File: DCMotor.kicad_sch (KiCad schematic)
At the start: 18 parts, among them J10 Conn_01x03_Socket, J11 Conn_01x02_Socket, J12 Conn_01x03_Socket, J13 Conn_01x03_Socket, J14 Conn_01x03_Socket, J7 Conn_01x02_Socket, J8 Conn_01x03_Socket, J9 Conn_01x02_Socket

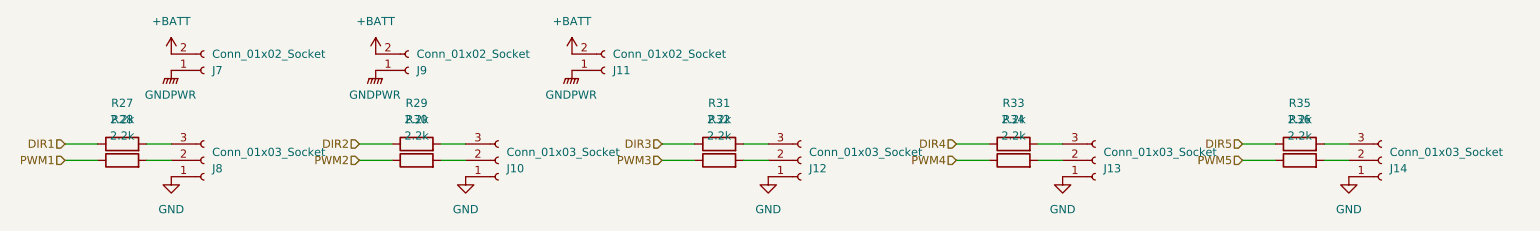
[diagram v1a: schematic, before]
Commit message: before elimination of J7
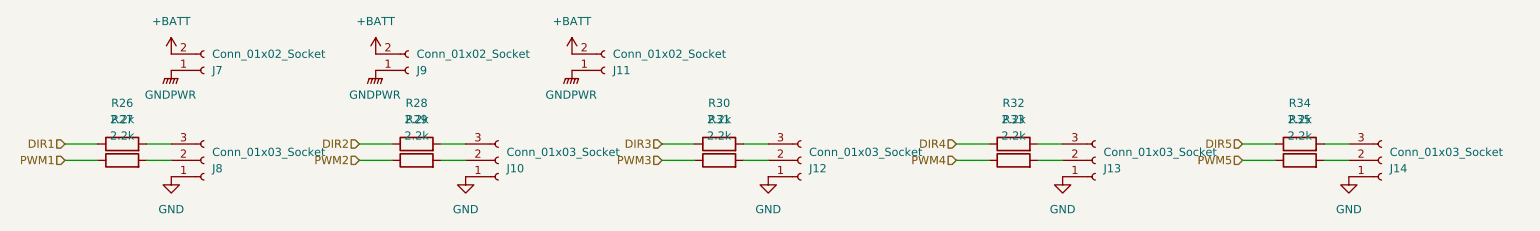
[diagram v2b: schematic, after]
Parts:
- renumbered R27 to R26, R28 to R27, R29 to R28, R30 to R29, R31 to R30, R32 to R31, R33 to R32, R34 to R33, R35 to R34, R36 to R35
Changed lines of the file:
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@@
 		(dnp no)
 		(fields_autoplaced yes)
-		(property "Reference" "R34"
+		(property "Reference" "R33"
 			(at 171.45 52.07 90)
 			(effects
@@
 			(project "chibarobo_board_2024"
 				(path "/7933aef9-9608-4ce1-b0d8-a4ffd3b998e4/10a4ce65-96c0-4b0e-ad7d-0749d3a88abd"
-					(reference "R34")
+					(reference "R33")
 					(unit 1)
 				)
@@
 		(dnp no)
 		(fields_autoplaced yes)
-		(property "Reference" "#PWR055"
+		(property "Reference" "#PWR054"
 			(at 72.39 49.53 0)
 			(effects
@@
 			(project "chibarobo_board_2024"
 				(path "/7933aef9-9608-4ce1-b0d8-a4ffd3b998e4/10a4ce65-96c0-4b0e-ad7d-0749d3a88abd"
-					(reference "#PWR055")
+					(reference "#PWR054")
 					(unit 1)
 				)
@@
 		(dnp no)
 		(fields_autoplaced yes)
-		(property "Reference" "#PWR052"
+		(property "Reference" "#PWR051"
 			(at 40.64 49.53 0)
 			(effects
@@
 			(project ""
 				(path "/7933aef9-9608-4ce1-b0d8-a4ffd3b998e4/10a4ce65-96c0-4b0e-ad7d-0749d3a88abd"
-					(reference "#PWR052")
+					(reference "#PWR051")
 					(unit 1)
 				)
@@
 		(dnp no)
 		(fields_autoplaced yes)
-		(property "Reference" "#PWR051"
+		(property "Reference" "#PWR050"
 			(at 40.64 45.72 0)
 			(effects
@@
 			(project ""
 				(path "/7933aef9-9608-4ce1-b0d8-a4ffd3b998e4/10a4ce65-96c0-4b0e-ad7d-0749d3a88abd"
-					(reference "#PWR051")
+					(reference "#PWR050")
 					(unit 1)
 				)
@@
 		(dnp no)
 		(fields_autoplaced yes)
-		(property "Reference" "R32"
+		(property "Reference" "R31"
 			(at 125.73 52.07 90)
 			(effects
@@
 			(project "chibarobo_board_2024"
 				(path "/7933aef9-9608-4ce1-b0d8-a4ffd3b998e4/10a4ce65-96c0-4b0e-ad7d-0749d3a88abd"
-					(reference "R32")
+					(reference "R31")
 					(unit 1)
 				)
@@
 		(dnp no)
 		(fields_autoplaced yes)
-		(property "Reference" "R31"
+		(property "Reference" "R30"
 			(at 125.73 49.53 90)
 			(effects
@@
 			(project "chibarobo_board_2024"
 				(path "/7933aef9-9608-4ce1-b0d8-a4ffd3b998e4/10a4ce65-96c0-4b0e-ad7d-0749d3a88abd"
-					(reference "R31")
+					(reference "R30")
 					(unit 1)
 				)
@@
 		(dnp no)
 		(fields_autoplaced yes)
-		(property "Reference" "R36"
+		(property "Reference" "R35"
 			(at 215.9 52.07 90)
 			(effects
@@
 			(project "chibarobo_board_2024"
 				(path "/7933aef9-9608-4ce1-b0d8-a4ffd3b998e4/10a4ce65-96c0-4b0e-ad7d-0749d3a88abd"
-					(reference "R36")
+					(reference "R35")
 					(unit 1)
 				)
@@
 		(dnp no)
 		(fields_autoplaced yes)
-		(property "Reference" "R33"
+		(property "Reference" "R32"
 			(at 171.45 49.53 90)
 			(effects
@@
 			(project "chibarobo_board_2024"
 				(path "/7933aef9-9608-4ce1-b0d8-a4ffd3b998e4/10a4ce65-96c0-4b0e-ad7d-0749d3a88abd"
-					(reference "R33")
+					(reference "R32")
 					(unit 1)
 				)
@@
 		(dnp no)
 		(fields_autoplaced yes)
-		(property "Reference" "R30"
+		(property "Reference" "R29"
 			(at 78.74 52.07 90)
 			(effects
@@
 			(project "chibarobo_board_2024"
 				(path "/7933aef9-9608-4ce1-b0d8-a4ffd3b998e4/10a4ce65-96c0-4b0e-ad7d-0749d3a88abd"
-					(reference "R30")
+					(reference "R29")
 					(unit 1)
 				)
@@
 		(dnp no)
 		(fields_autoplaced yes)
-		(property "Reference" "R35"
+		(property "Reference" "R34"
 			(at 215.9 49.53 90)
 			(effects
@@
 			(project "chibarobo_board_2024"
 				(path "/7933aef9-9608-4ce1-b0d8-a4ffd3b998e4/10a4ce65-96c0-4b0e-ad7d-0749d3a88abd"
-					(reference "R35")
+					(reference "R34")
 					(unit 1)
 				)
@@
 		(dnp no)
 		(fields_autoplaced yes)
-		(property "Reference" "#PWR057"
+		(property "Reference" "#PWR056"
 			(at 102.87 45.72 0)
 			(effects
@@
 			(project ""
 				(path "/7933aef9-9608-4ce1-b0d8-a4ffd3b998e4/10a4ce65-96c0-4b0e-ad7d-0749d3a88abd"
-					(reference "#PWR057")
+					(reference "#PWR056")
 					(unit 1)
 				)
@@
 		(dnp no)
 		(fields_autoplaced yes)
-		(property "Reference" "#PWR060"
+		(property "Reference" "#PWR059"
 			(at 179.07 67.31 0)
 			(effects
@@
 			(project "chibarobo_board_2024"
 				(path "/7933aef9-9608-4ce1-b0d8-a4ffd3b998e4/10a4ce65-96c0-4b0e-ad7d-0749d3a88abd"
-					(reference "#PWR060")
+					(reference "#PWR059")
 					(unit 1)
 				)
@@
 		(dnp no)
 		(fields_autoplaced yes)
-		(property "Reference" "#PWR058"
+		(property "Reference" "#PWR057"
 			(at 102.87 49.53 0)
 			(effects
@@
 			(project "chibarobo_board_2024"
 				(path "/7933aef9-9608-4ce1-b0d8-a4ffd3b998e4/10a4ce65-96c0-4b0e-ad7d-0749d3a88abd"
-					(reference "#PWR058")
+					(reference "#PWR057")
 					(unit 1)
 				)
@@
 		(dnp no)
 		(fields_autoplaced yes)
-		(property "Reference" "#PWR054"
+		(property "Reference" "#PWR053"
 			(at 72.39 45.72 0)
 			(effects
@@
 			(project ""
 				(path "/7933aef9-9608-4ce1-b0d8-a4ffd3b998e4/10a4ce65-96c0-4b0e-ad7d-0749d3a88abd"
-					(reference "#PWR054")
+					(reference "#PWR053")
 					(unit 1)
 				)
@@
 		(dnp no)
 		(fields_autoplaced yes)
-		(property "Reference" "#PWR056"
+		(property "Reference" "#PWR055"
 			(at 86.36 67.31 0)
 			(effects
@@
 			(project "chibarobo_board_2024"
 				(path "/7933aef9-9608-4ce1-b0d8-a4ffd3b998e4/10a4ce65-96c0-4b0e-ad7d-0749d3a88abd"
-					(reference "#PWR056")
+					(reference "#PWR055")
 					(unit 1)
 				)
@@
 		(dnp no)
 		(fields_autoplaced yes)
-		(property "Reference" "#PWR061"
+		(property "Reference" "#PWR060"
 			(at 223.52 67.31 0)
 			(effects
@@
 			(project "chibarobo_board_2024"
 				(path "/7933aef9-9608-4ce1-b0d8-a4ffd3b998e4/10a4ce65-96c0-4b0e-ad7d-0749d3a88abd"
-					(reference "#PWR061")
+					(reference "#PWR060")
 					(unit 1)
 				)
@@
 		(dnp no)
 		(fields_autoplaced yes)
-		(property "Reference" "#PWR053"
+		(property "Reference" "#PWR052"
 			(at 40.64 67.31 0)
 			(effects
@@
 			(project ""
 				(path "/7933aef9-9608-4ce1-b0d8-a4ffd3b998e4/10a4ce65-96c0-4b0e-ad7d-0749d3a88abd"
-					(reference "#PWR053")
+					(reference "#PWR052")
 					(unit 1)
 				)
@@
 		(dnp no)
 		(fields_autoplaced yes)
-		(property "Reference" "R27"
+		(property "Reference" "R26"
 			(at 33.02 49.53 90)
 			(effects
@@
 			(project ""
 				(path "/7933aef9-9608-4ce1-b0d8-a4ffd3b998e4/10a4ce65-96c0-4b0e-ad7d-0749d3a88abd"
-					(reference "R27")
+					(reference "R26")
 					(unit 1)
 				)
@@
 		(dnp no)
 		(fields_autoplaced yes)
-		(property "Reference" "R29"
+		(property "Reference" "R28"
 			(at 78.74 49.53 90)
 			(effects
@@
 			(project "chibarobo_board_2024"
 				(path "/7933aef9-9608-4ce1-b0d8-a4ffd3b998e4/10a4ce65-96c0-4b0e-ad7d-0749d3a88abd"
-					(reference "R29")
+					(reference "R28")
 					(unit 1)
 				)
@@
 		(dnp no)
 		(fields_autoplaced yes)
-		(property "Reference" "R28"
+		(property "Reference" "R27"
 			(at 33.02 52.07 90)
 			(effects
@@
 			(project ""
 				(path "/7933aef9-9608-4ce1-b0d8-a4ffd3b998e4/10a4ce65-96c0-4b0e-ad7d-0749d3a88abd"
-					(reference "R28")
+					(reference "R27")
 					(unit 1)
 				)
@@
 		(dnp no)
 		(fields_autoplaced yes)
-		(property "Reference" "#PWR059"
+		(property "Reference" "#PWR058"
 			(at 133.35 67.31 0)
 			(effects
@@
 			(project "chibarobo_board_2024"
 				(path "/7933aef9-9608-4ce1-b0d8-a4ffd3b998e4/10a4ce65-96c0-4b0e-ad7d-0749d3a88abd"
-					(reference "#PWR059")
-					(unit 1)
-				)
+					(reference "#PWR058")
+					(unit 1)
+				)
